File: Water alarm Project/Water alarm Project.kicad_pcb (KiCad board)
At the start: 2 copper layers, 39.1 x 38.8 mm, 13 parts, among them J1 Jack-DC, J2 Screw_Terminal_01x02, Q1 2N7000

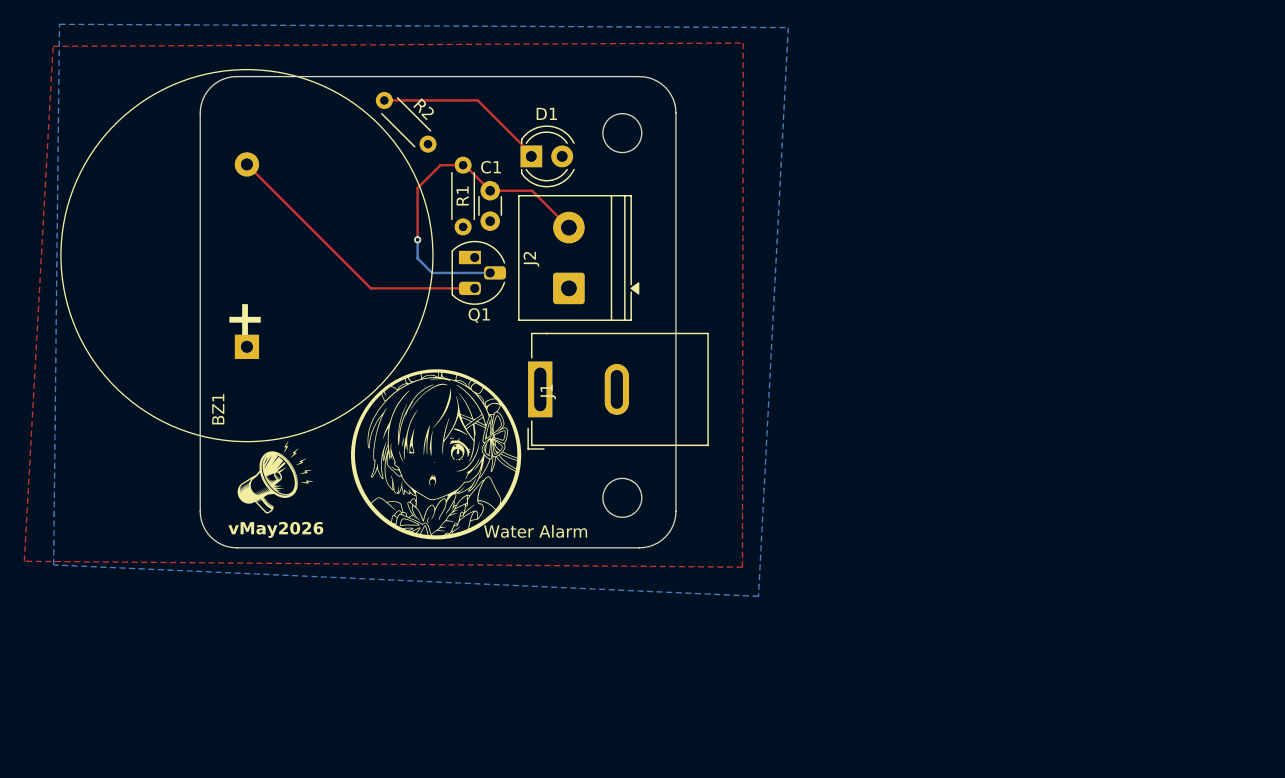
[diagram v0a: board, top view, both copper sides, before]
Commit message: Modified gerber files and pngs
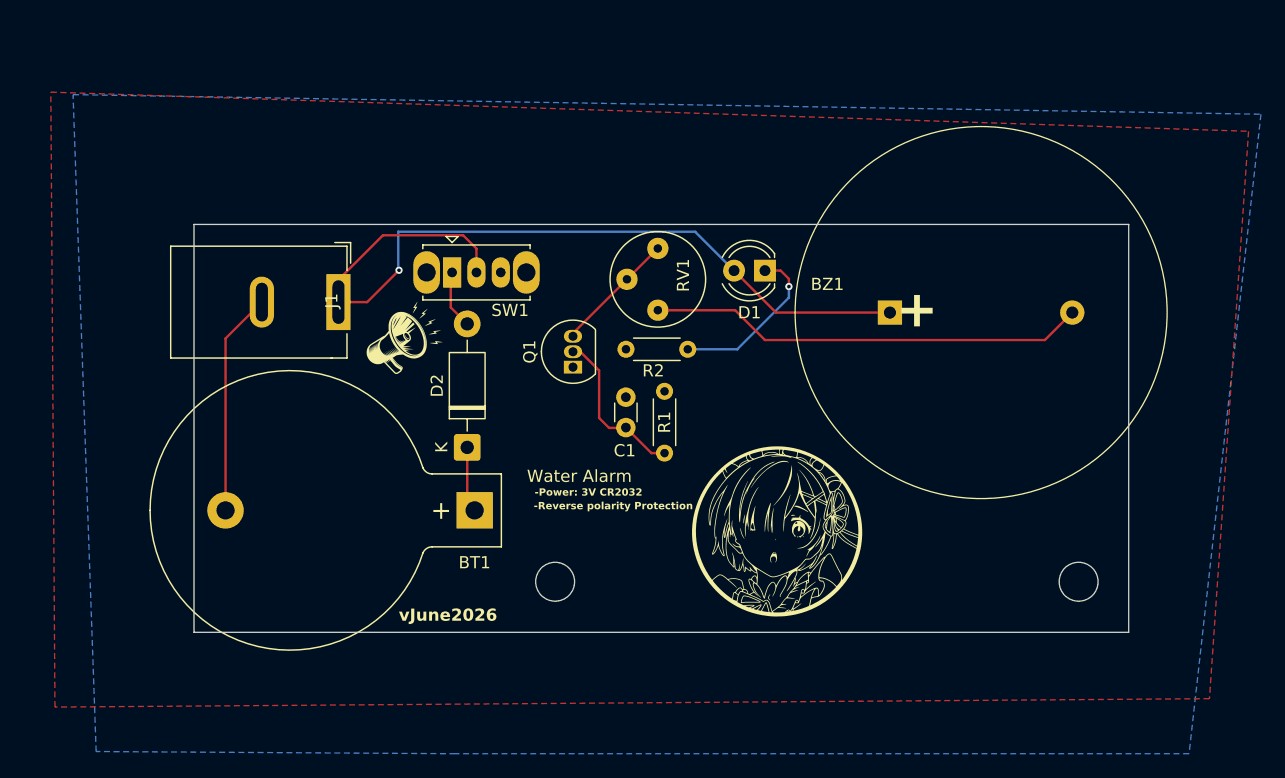
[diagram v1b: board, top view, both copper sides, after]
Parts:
- removed the G*** at (158.7, 122.8)
- removed J2: Screw_Terminal_01x02, TerminalBlock_Phoenix:TerminalBlock_Phoenix_PT-1,5-2-5.0-H_1x02_P5.00mm_Horizontal
- added BT1: Battery_Cell, Battery:BatteryHolder_Keystone_103_1x20mm, F.Cu at (175.5, 125.3)
- added D2: 1N4007, Diode_THT:D_DO-41_SOD81_P10.16mm_Horizontal, F.Cu at (174.9, 120.1)
- added RV1: 1k, Potentiometer_THT:Potentiometer_Bourns_3339P_Vertical_HandSoldering, F.Cu at (190.6, 108.8)
- added SW1: SW_SPDT, Button_Switch_THT:SW_Slide_SPDT_Straight_CK_OS102011MS2Q, F.Cu at (173.7, 105.7)
- G***: moved to F.Cu
- Q1: footprint Package_TO_SOT_THT:TO-92L_HandSolder -> Package_TO_SOT_THT:TO-92_Inline
- R2: value 6.8k -> 200
- moved BZ1 60.6 mm to (217.2, 109.0), turned to 0 degrees
- moved REF** 38.2 mm to (225.2, 131.2), turned to 180 degrees
- moved REF** 37.3 mm to (182.1, 131.2)
- moved R2 32.3 mm to (193.0, 112.0), turned to 180 degrees
- moved R1 28.9 mm to (191.1, 120.6), turned to 90 degrees
- moved G*** 28.8 mm to (200.4, 127.0)
- moved C1 22.5 mm to (187.9, 118.5), turned to 90 degrees
- moved D1 21.4 mm to (199.4, 105.6), turned to 180 degrees
- moved J1 18.1 mm to (164.3, 108.2), turned to -90 degrees
- moved G*** 15.8 mm to (169.3, 111.4), turned to 0 degrees
- moved Q1 12.1 mm to (183.6, 113.5), turned to 90 degrees
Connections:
- Q1 pad 3: Net-(BZ1--) -> Net-(Q1-D)
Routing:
- net VCC: track 0.00 -> 69.6 mm, vias 0 -> 1
- net GND: track 0.29 -> 18.4 mm
- net /Gate: track 27.6 -> 13.3 mm, vias 1 -> 0
- net Net-(BZ1--): track 23.0 -> 36.0 mm
- net Net-(Q1-D): track 0.00 -> 10.1 mm
- net Net-(BT1-+): track 0.00 -> 5.43 mm
- net Net-(D2-A): track 0.00 -> 4.83 mm
- net Net-(D1-K): track 14.4 -> 13.9 mm, vias 0 -> 1
- added copper zone on B.Cu, net GND
- added copper zone on F.Cu, net VCC
- removed copper zone on F.Cu, net GND
- removed copper zone on B.Cu, net VCC
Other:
- board size 39.1 x 38.8 mm -> 76.9 x 33.6 mm
- board text added: "-Power: 3V CR2032"
- board text added: "-Reverse polarity Protection"
- board text added: "vJune2026"
- board text removed: "vMay2026"
